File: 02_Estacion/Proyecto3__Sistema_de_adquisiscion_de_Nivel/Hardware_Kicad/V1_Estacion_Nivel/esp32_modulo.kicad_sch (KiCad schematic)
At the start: 17 parts, among them J10 M20-9991045, J7 M20-9990245, SW1 RST, SW3 BOOT, U2 ESP32-S3-WROOM-1-N16R8

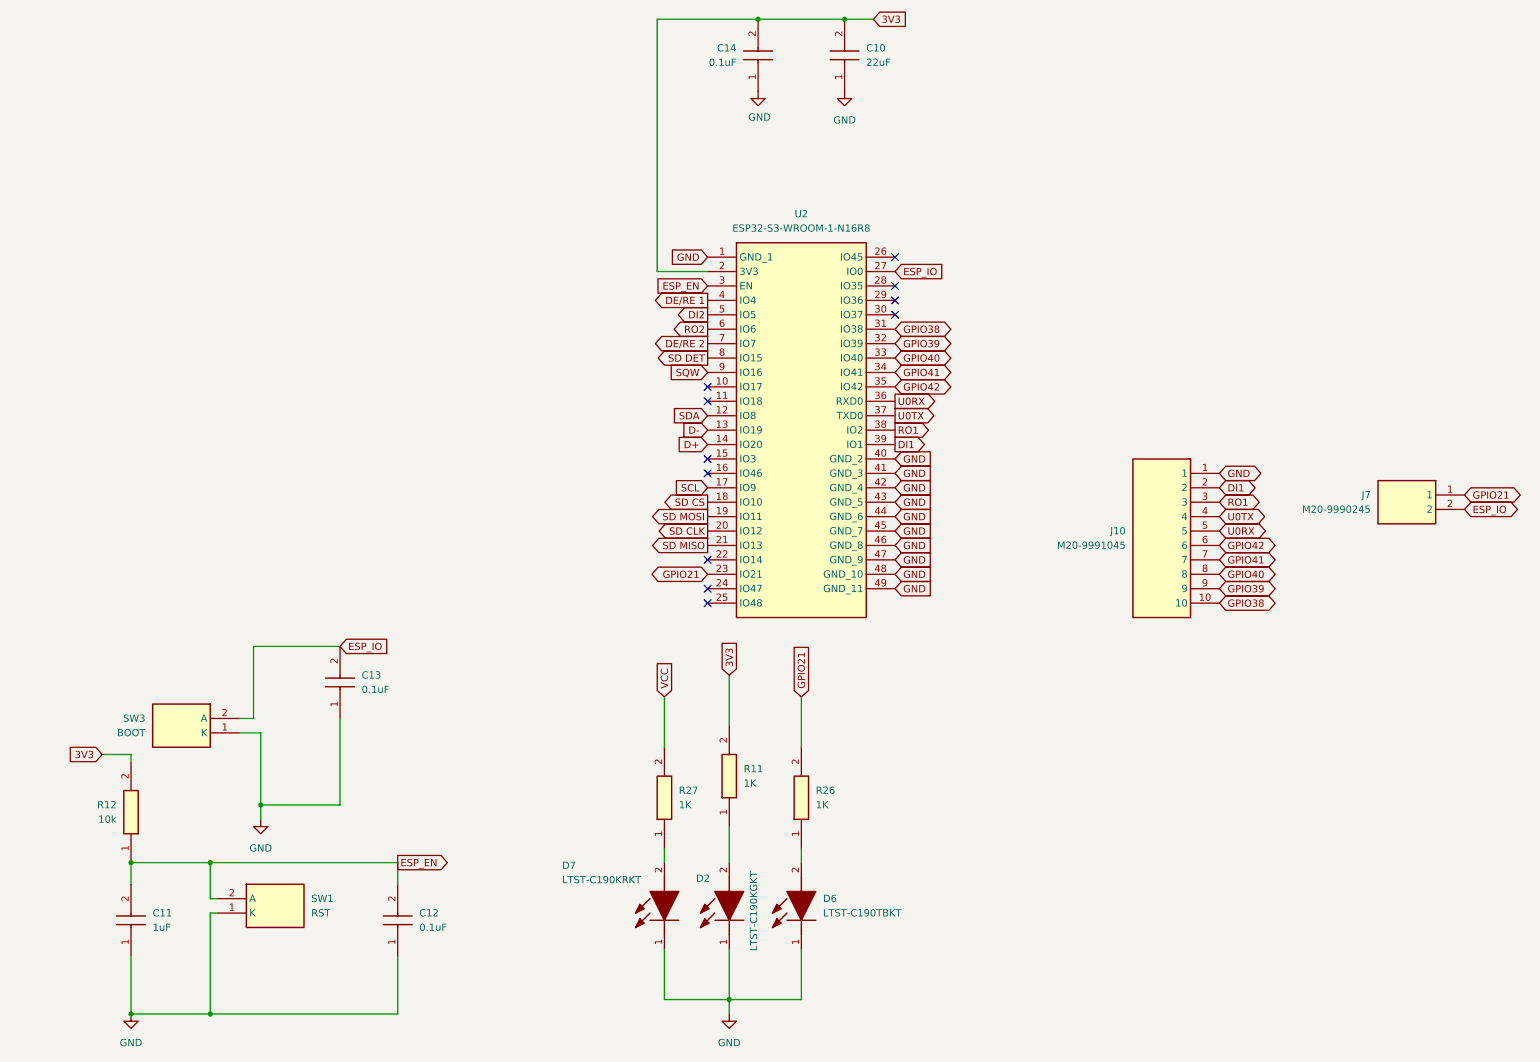
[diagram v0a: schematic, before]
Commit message: update
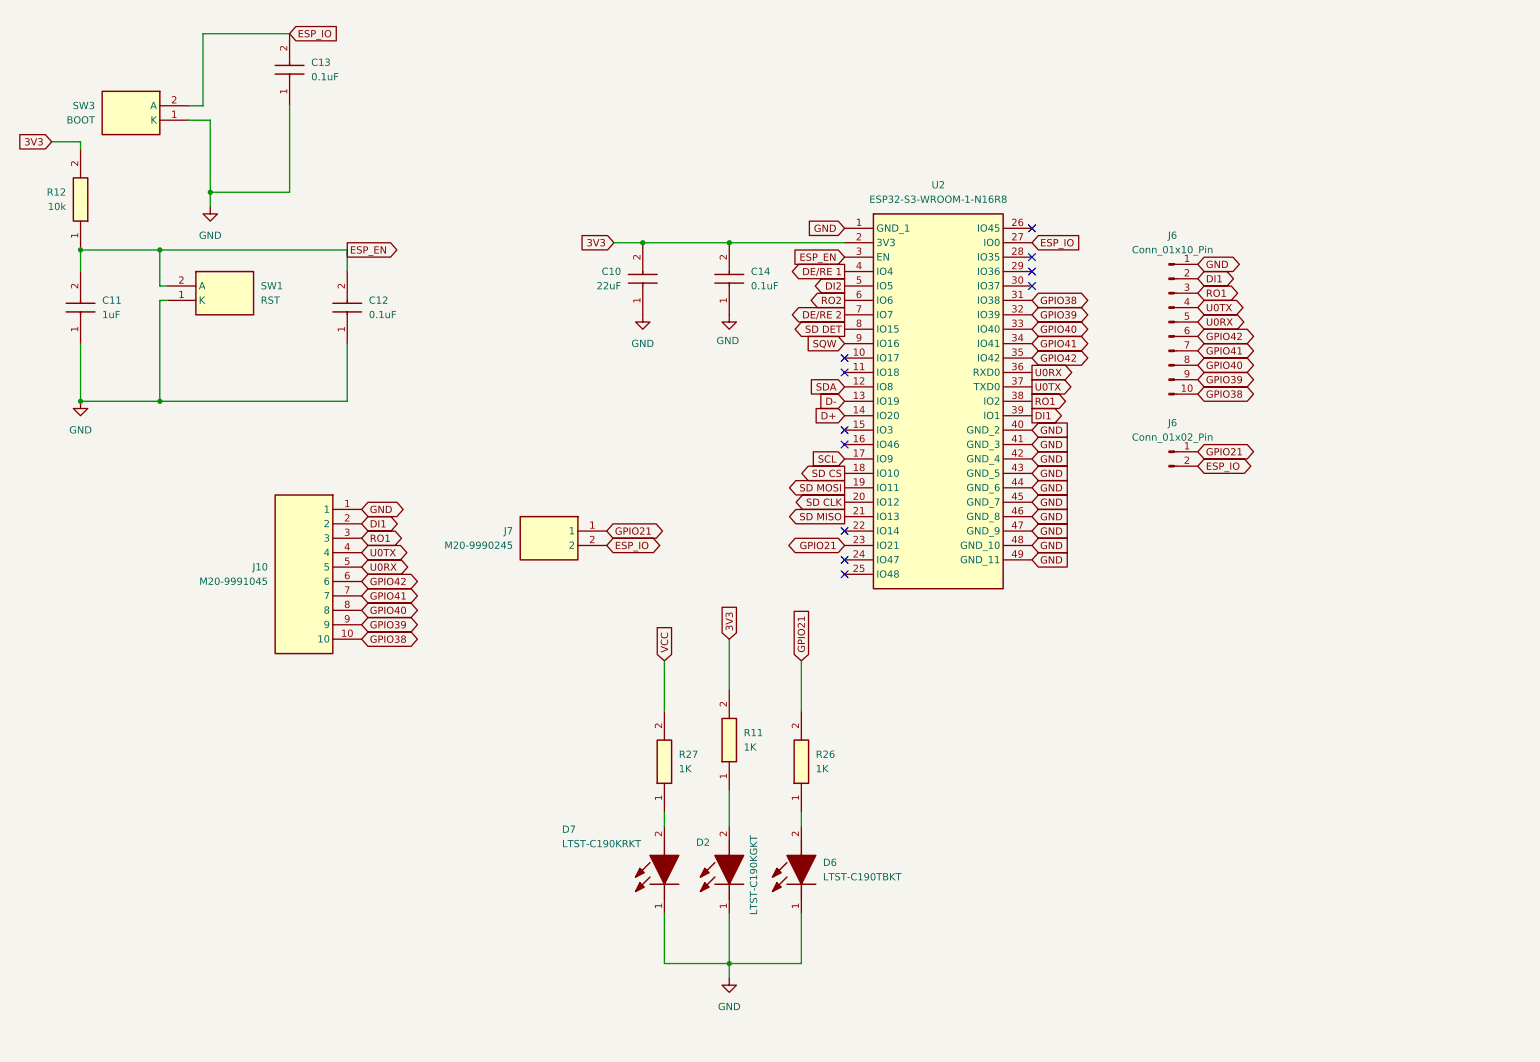
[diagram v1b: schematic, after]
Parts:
- added J6: Conn_01x02_Pin, Connector_PinHeader_2.54mm:PinHeader_1x02_P2.54mm_Vertical, symbol Connector:Conn_01x02_Pin
- added J6: Conn_01x10_Pin, Connector_PinHeader_2.54mm:PinHeader_1x10_P2.54mm_Vertical, symbol Connector:Conn_01x10_Pin
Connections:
- net DI1: now also J6.2 (Pin_2)
- net ESP_IO: now also J6.2 (Pin_2)
- net GND: now also J6.1 (Pin_1)
- net GPIO21: now also J6.1 (Pin_1)
- net GPIO38: now also J6.10 (Pin_10)
- net GPIO39: now also J6.9 (Pin_9)
- net GPIO40: now also J6.8 (Pin_8)
- net GPIO41: now also J6.7 (Pin_7)
- net GPIO42: now also J6.6 (Pin_6)
- net RO1: now also J6.3 (Pin_3)
- net U0RX: now also J6.5 (Pin_5)
- net U0TX: now also J6.4 (Pin_4)
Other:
- moved on the sheet: C10, C11, C12, C13, C14, D2, D6, D7, J10, J7, R11, R12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
